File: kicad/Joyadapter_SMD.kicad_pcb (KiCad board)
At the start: 2 copper layers, 47 x 37 mm, 18 parts, among them J1 AVR-ISP-6, J3 USB_B_Mini, U1 ATtiny4313-SU, X1 DB9_male, X2 DB9_male, Y1 12MHz

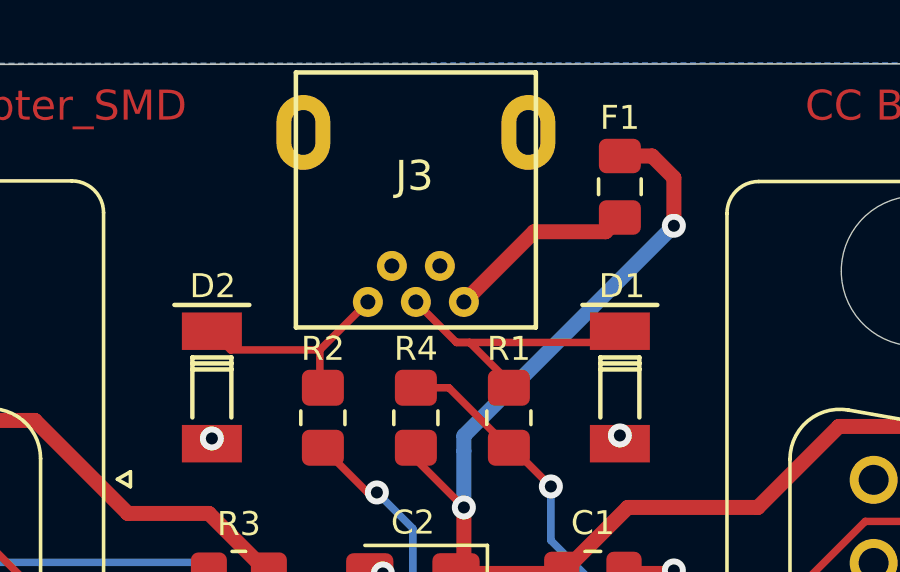
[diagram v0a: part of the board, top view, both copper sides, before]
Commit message: Update PCB to V1.0
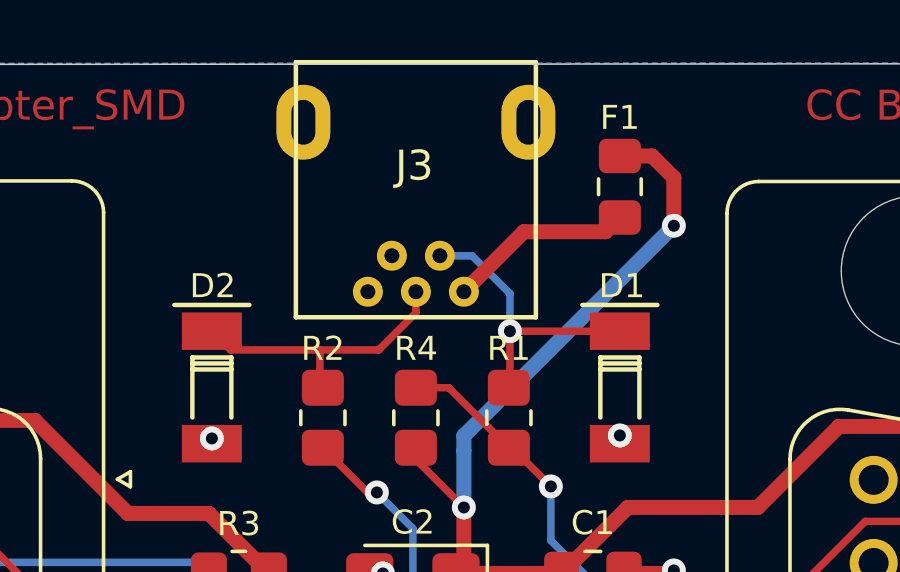
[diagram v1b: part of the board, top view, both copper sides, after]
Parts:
- moved J3 0.34 mm to (149.2, 90.2)
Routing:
- net /D+: track 7.42 -> 9.57 mm
- net /D-: track 9.81 -> 10.2 mm, vias 0 -> 1
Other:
- board text added: "V1.0 - 06/21 - der-pw https://github.com/der-pw/USB-Joyadapter_SMD"
- board text removed: "V0.9 - 01/21 - der-pw https://github.com/der-pw/USB-Joyadapter_SMD"
